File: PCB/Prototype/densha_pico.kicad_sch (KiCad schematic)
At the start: 33 parts, among them J1 NV3007, J2 Conn_01x04, J3 Conn_01x02, J4 NV3007_Stub, J5 Spin, J6 Spin, Q1 AO3400A, U1 PiPico_No_SWD, U2 CH221K, U3 DC/DC, U4 TMC2209, U5 8002A_Tap, U6 AS5600

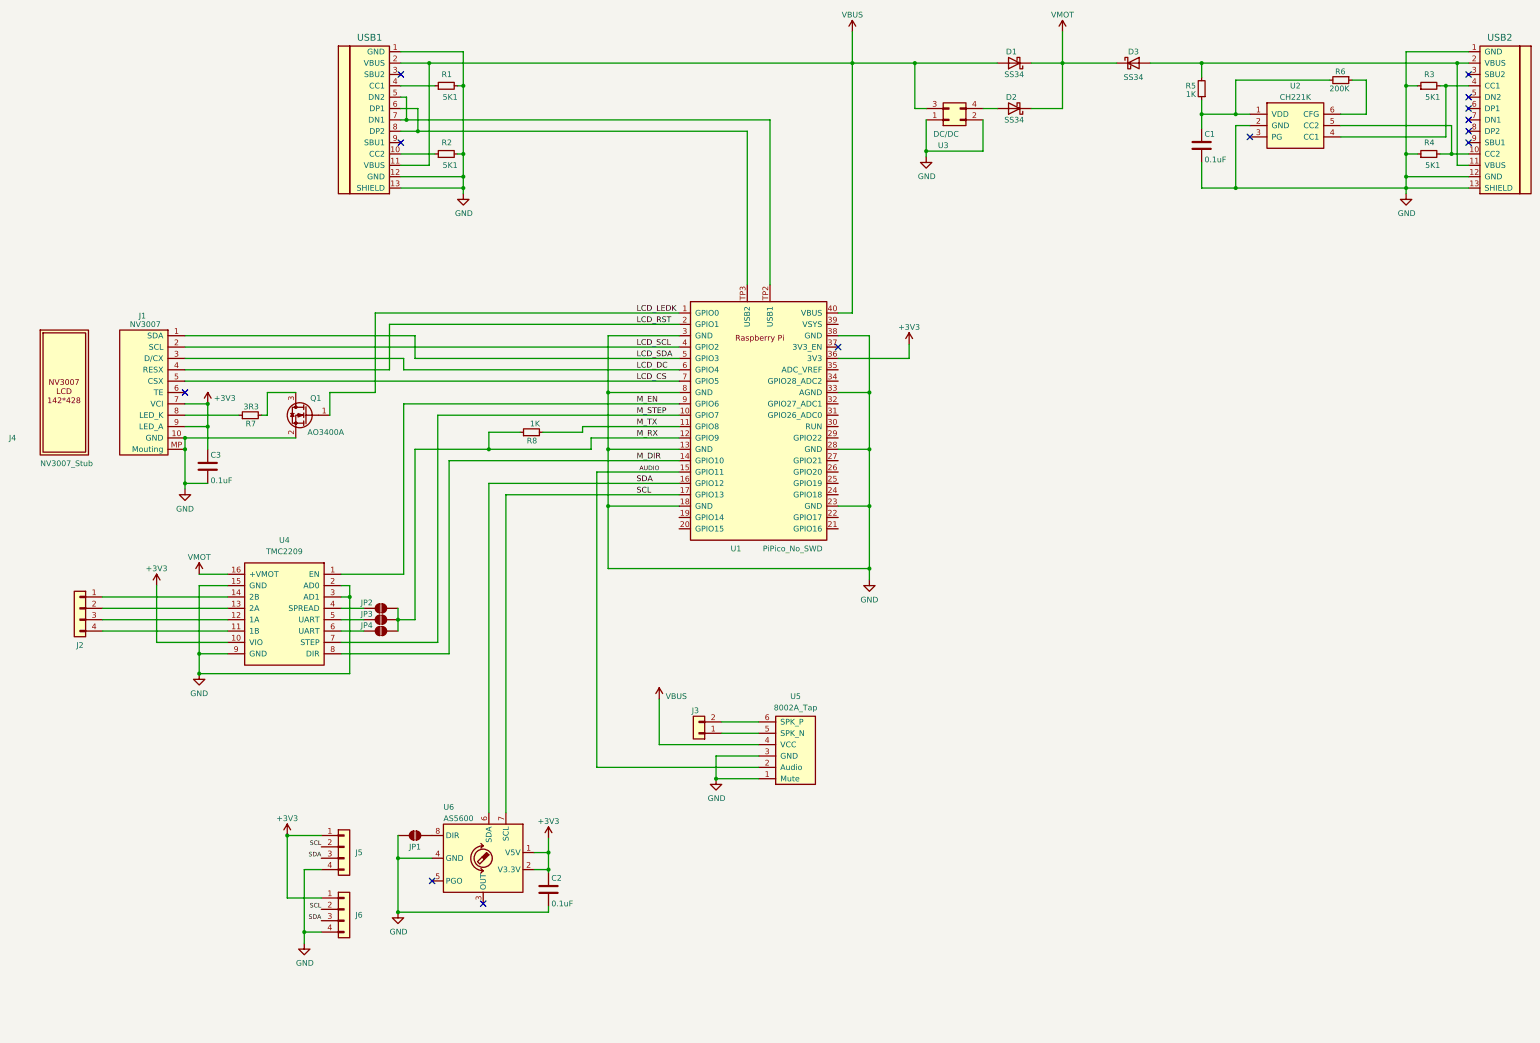
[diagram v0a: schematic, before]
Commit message: PCB v0.3
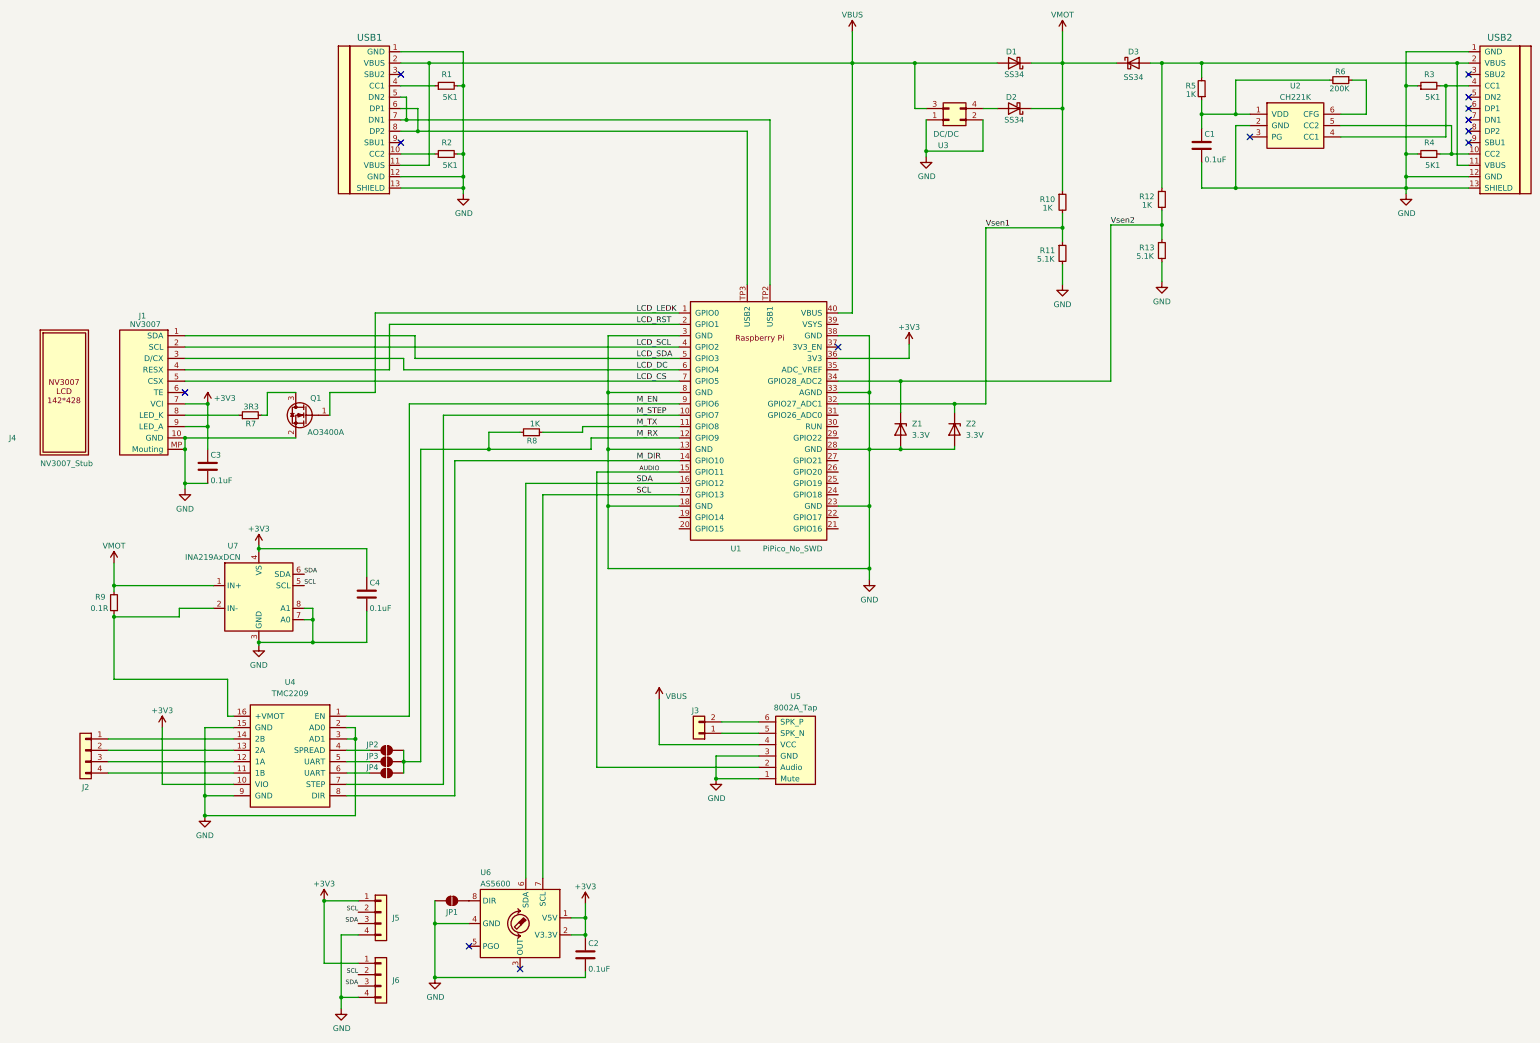
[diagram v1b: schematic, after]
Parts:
- added C4: 0.1uF, Capacitor_SMD:C_0603_1608Metric_Pad1.08x0.95mm_HandSolder, symbol Device:C
- added R10, R12: 1K, Resistor_SMD:R_0603_1608Metric_Pad0.98x0.95mm_HandSolder, symbol Device:R_Small
- added R11, R13: 5.1K, Resistor_SMD:R_0603_1608Metric_Pad0.98x0.95mm_HandSolder, symbol Device:R_Small
- added R9: 0.1R, Inductor_SMD:L_1206_3216Metric_Pad1.42x1.75mm_HandSolder, symbol Device:R_Small
- added U7: INA219AxDCN, densha_pico:SOT-23-8_Thin, symbol Sensor_Energy:INA219AxDCN
- added Z1, Z2: 3.3V, Diode_SMD:D_SOD-123F, symbol Device:D_Zener
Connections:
- net +3V3: now also C4.1, U7.4 (VS)
- net GND: now also C4.2, R11.2, R13.2, U7.3 (GND), U7.7 (A0), U7.8 (A1), Z1.2 (A), Z2.2 (A)
- net SCL: now also U7.5 (SCL)
- net SDA: now also U7.6 (SDA)
- net VMOT: now also R10.1, R9.2, U7.1 (IN+); no longer U4.16 (+VMOT)
- net at D3.2 (A), R5.2, USB2.11 (VBUS)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: now also R12.1
- net Vsen1: now reaches U1.32 (GPIO27_ADC1)
- net Vsen1: now also R10.2, R11.1, Z2.1 (K)
- net Vsen2: now reaches U1.34 (GPIO28_ADC2)
- net Vsen2: now also R12.2, R13.1, Z1.1 (K)
- new net: R9.1, U4.16 (+VMOT), U7.2 (IN-)
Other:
- moved on the sheet: C2, J2, J5, J6, JP1, JP2, JP3, JP4, U4, U6
